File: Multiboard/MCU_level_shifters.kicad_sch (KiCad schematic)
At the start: 45 parts, among them Q1 Q_Dual_NMOS_G1S2G2D2S1D1, Q14 Q_Dual_NMOS_G1S2G2D2S1D1, Q2 Q_Dual_NMOS_G1S2G2D2S1D1, Q3 Q_Dual_NMOS_G1S2G2D2S1D1, Q4 Q_Dual_NMOS_G1S2G2D2S1D1, Q5 Q_Dual_NMOS_G1S2G2D2S1D1, Q6 Q_Dual_NMOS_G1S2G2D2S1D1, Q7 Q_Dual_NMOS_G1S2G2D2S1D1, SW3 SW_SPST, SW4 SW_SPST, SW5 SW_SPST, SW7 SW_SPST, SW9 SW_SPST

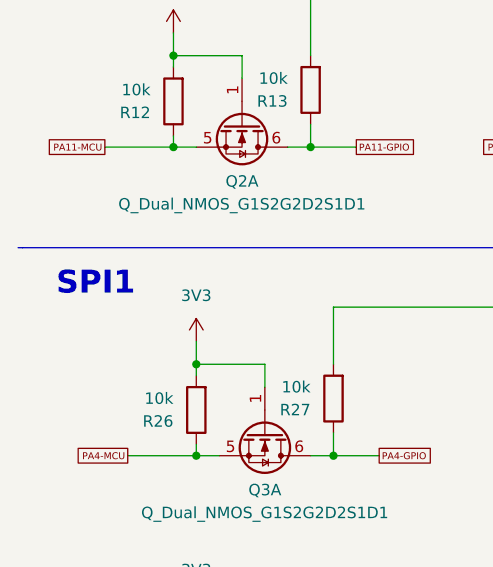
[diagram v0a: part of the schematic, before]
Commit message: Fixed bus implementation
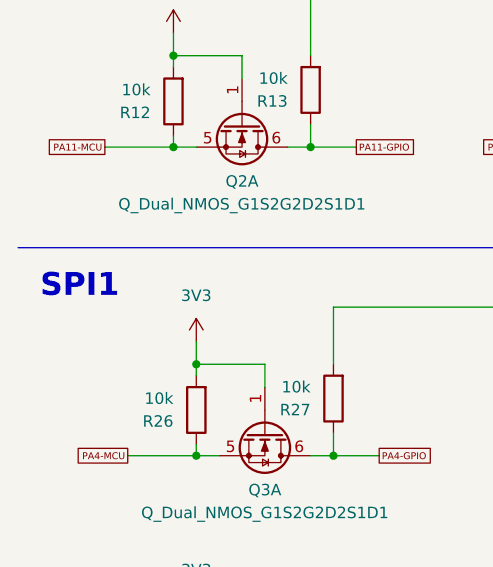
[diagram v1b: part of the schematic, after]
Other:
- moved on the sheet: Q2A
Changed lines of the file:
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@@
 	(text "SPI1"
 		(exclude_from_sim no)
-		(at 20.574 106.68 0)
+		(at 18.796 106.934 0)
 		(effects
 			(font
@@
 	(symbol
 		(lib_id "Transistor_FET:Q_Dual_NMOS_G1S2G2D2S1D1")
-		(at 85.09 88.9 270)
-		(unit 2)
+		(at 36.83 88.9 270)
+		(unit 1)
 		(exclude_from_sim no)
 		(in_bom yes)
@@
 		(fields_autoplaced yes)
 		(property "Reference" "Q2"
-			(at 85.09 95.25 90)
+			(at 36.83 95.25 90)
 			(effects
 				(font
@@
 		)
 		(property "Value" "Q_Dual_NMOS_G1S2G2D2S1D1"
-			(at 85.09 97.79 90)
+			(at 36.83 97.79 90)
 			(effects
 				(font
@@
 		)
 		(property "Footprint" "Package_SO:SOIC-8_3.9x4.9mm_P1.27mm"
-			(at 85.09 93.98 0)
+			(at 36.83 93.98 0)
 			(effects
 				(font
@@
 		)
 		(property "Datasheet" "~"
-			(at 85.09 93.98 0)
+			(at 36.83 93.98 0)
 			(effects
 				(font
@@
 		)
 		(property "Description" "Dual NMOS transistor, 6 pin package"
-			(at 85.09 88.9 0)
+			(at 36.83 88.9 0)
 			(effects
 				(font
@@
 				(path "/9ed4a389-3aa7-41f1-b239-280eb7f09ef1/47d00c33-b241-4dd6-bf0c-4e5c6f2dc35e"
 					(reference "Q2")
-					(unit 2)
+					(unit 1)
 				)
 			)
@@
 	(symbol
 		(lib_id "Transistor_FET:Q_Dual_NMOS_G1S2G2D2S1D1")
-		(at 36.83 88.9 270)
-		(unit 1)
+		(at 85.09 88.9 270)
+		(unit 2)
 		(exclude_from_sim no)
 		(in_bom yes)
@@
 		(fields_autoplaced yes)
 		(property "Reference" "Q2"
-			(at 36.83 95.25 90)
+			(at 85.09 95.25 90)
 			(effects
 				(font
@@
 		)
 		(property "Value" "Q_Dual_NMOS_G1S2G2D2S1D1"
-			(at 36.83 97.79 90)
+			(at 85.09 97.79 90)
 			(effects
 				(font
@@
 		)
 		(property "Footprint" "Package_SO:SOIC-8_3.9x4.9mm_P1.27mm"
-			(at 36.83 93.98 0)
+			(at 85.09 93.98 0)
 			(effects
 				(font
@@
 		)
 		(property "Datasheet" "~"
-			(at 36.83 93.98 0)
+			(at 85.09 93.98 0)
 			(effects
 				(font
@@
 		)
 		(property "Description" "Dual NMOS transistor, 6 pin package"
-			(at 36.83 88.9 0)
+			(at 85.09 88.9 0)
 			(effects
 				(font
@@
 				(path "/9ed4a389-3aa7-41f1-b239-280eb7f09ef1/47d00c33-b241-4dd6-bf0c-4e5c6f2dc35e"
 					(reference "Q2")
-					(unit 1)
+					(unit 2)
 				)
 			)
